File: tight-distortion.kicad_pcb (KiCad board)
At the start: 2 copper layers, 60 x 80 mm, 4 parts, among them J1 Barrel_Jack_Switch, J2 AudioJack_TRS, J3 AudioJack_TRS

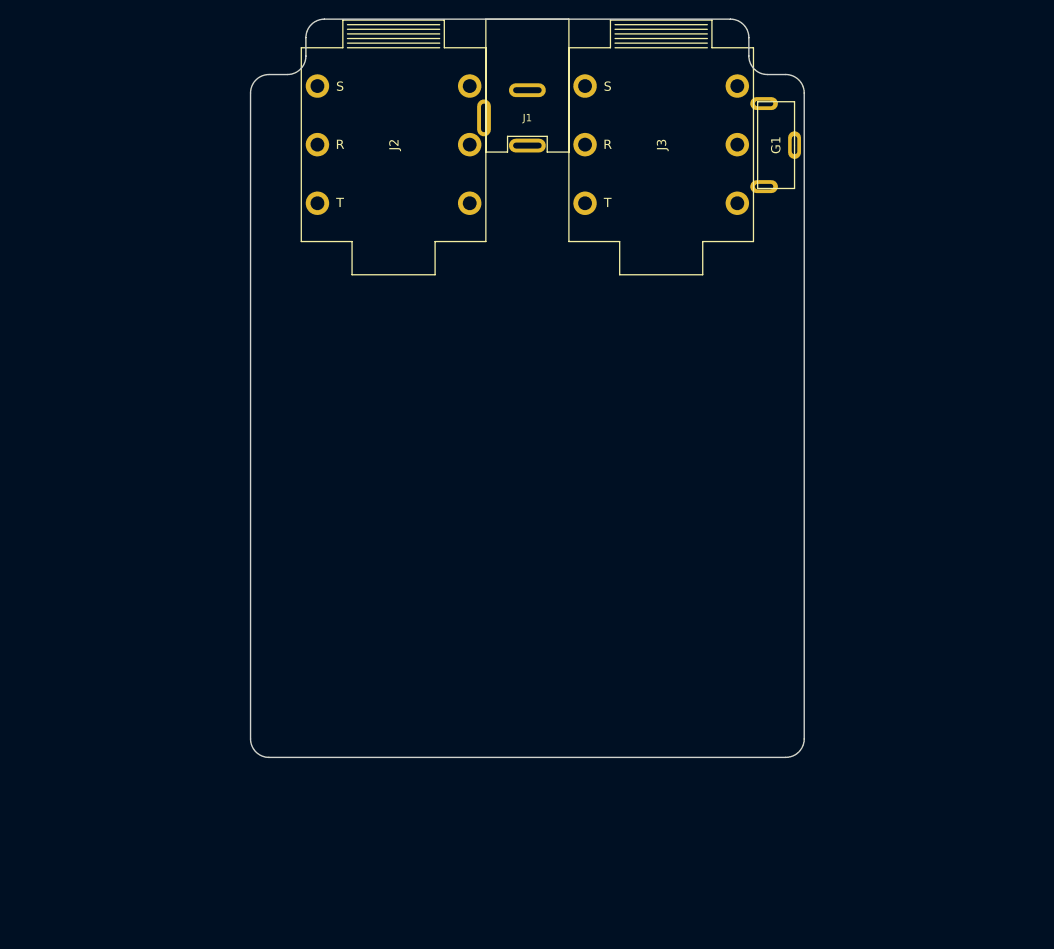
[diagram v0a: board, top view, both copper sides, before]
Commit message: first PCB layout draft
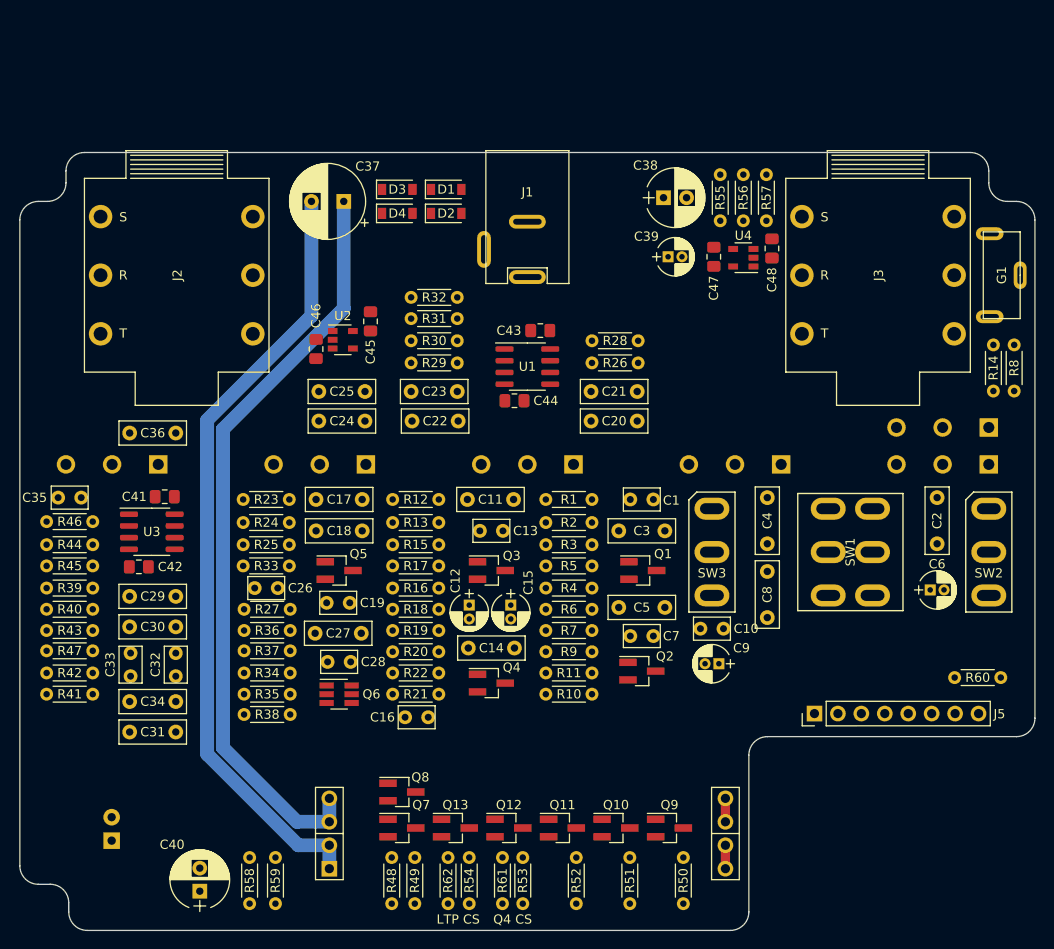
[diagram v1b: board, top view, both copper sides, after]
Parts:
- added C1: 220pF, bca-footprints:C_Ceramic_L4.0mm_W2.5mm_P2.50mm, F.Cu at (12.4, -5.70)
- added C10: 100pF, bca-footprints:C_Ceramic_L4.0mm_W2.5mm_P2.50mm, F.Cu at (20.0, 8.30)
- added C11: 2.2nF, bca-footprints:C_Film_L7.2mm_W2.5mm_P5.00mm, F.Cu at (-4.00, -5.70)
- added C12: 10uF, bca-footprints:CP_Radial_D4.0mm_P1.50mm, F.Cu at (-6.30, 6.50)
- added C13: 100pF, bca-footprints:C_Ceramic_L4.0mm_W2.5mm_P2.50mm, F.Cu at (-3.90, -2.30)
- added C14: 4.7nF, bca-footprints:C_Film_L7.2mm_W2.5mm_P5.00mm, F.Cu at (-3.90, 10.4)
- added C15: 10uF, bca-footprints:CP_Radial_D4.0mm_P1.50mm, F.Cu at (-1.80, 6.50)
- added C16: 100pF, bca-footprints:C_Ceramic_L4.0mm_W2.5mm_P2.50mm, F.Cu at (-12.0, 17.9)
- added C17: 0.1uF, bca-footprints:C_Film_L7.2mm_W2.5mm_P5.00mm, F.Cu at (-20.4, -5.70)
- added C18: 0.1uF, bca-footprints:C_Film_L7.2mm_W2.5mm_P5.00mm, F.Cu at (-20.4, -2.30)
- added C19: 100pF, bca-footprints:C_Ceramic_L4.0mm_W2.5mm_P2.50mm, F.Cu at (-20.5, 5.50)
- added C2: 10nF, bca-footprints:C_Film_L7.2mm_W2.5mm_P5.00mm, F.Cu at (44.4, -3.40)
- added C20: 10nF, bca-footprints:C_Film_L7.2mm_W2.5mm_P5.00mm, F.Cu at (9.40, -14.2)
- added C21: 10nF, bca-footprints:C_Film_L7.2mm_W2.5mm_P5.00mm, F.Cu at (9.40, -17.4)
- added C22: 10nF, bca-footprints:C_Film_L7.2mm_W2.5mm_P5.00mm, F.Cu at (-10.0, -14.2)
- added C23: 10nF, bca-footprints:C_Film_L7.2mm_W2.5mm_P5.00mm, F.Cu at (-10.1, -17.4)
- added C24: 10nF, bca-footprints:C_Film_L7.2mm_W2.5mm_P5.00mm, F.Cu at (-20.1, -14.2)
- added C25: 10nF, bca-footprints:C_Film_L7.2mm_W2.5mm_P5.00mm, F.Cu at (-20.1, -17.4)
- added C26: 100pF, bca-footprints:C_Ceramic_L4.0mm_W2.5mm_P2.50mm, F.Cu at (-28.3, 3.90)
- added C27: 10nF, bca-footprints:C_Film_L7.2mm_W2.5mm_P5.00mm, F.Cu at (-20.5, 8.80)
- added C28: 100pF, bca-footprints:C_Ceramic_L4.0mm_W2.5mm_P2.50mm, F.Cu at (-20.4, 11.9)
- added C29: 0.1uF, bca-footprints:C_Film_L7.2mm_W2.5mm_P5.00mm, F.Cu at (-40.6, 4.80)
- added C3: 1nF, bca-footprints:C_Film_L7.2mm_W2.5mm_P5.00mm, F.Cu at (12.4, -2.30)
- added C30: 0.1uF, bca-footprints:C_Film_L7.2mm_W2.5mm_P5.00mm, F.Cu at (-40.6, 8.10)
- added C31: 0.1uF, bca-footprints:C_Film_L7.2mm_W2.5mm_P5.00mm, F.Cu at (-40.6, 19.5)
- added C32: 270pF, bca-footprints:C_Ceramic_L4.0mm_W2.5mm_P2.50mm, F.Cu at (-38.1, 12.2)
- added C33: 270pF, bca-footprints:C_Ceramic_L4.0mm_W2.5mm_P2.50mm, F.Cu at (-43.0, 12.2)
- added C34: 3.3nF, bca-footprints:C_Film_L7.2mm_W2.5mm_P5.00mm, F.Cu at (-40.6, 16.2)
- added C35: 100pF, bca-footprints:C_Ceramic_L4.0mm_W2.5mm_P2.50mm, F.Cu at (-49.6, -5.90)
- added C36: 0.1uF, bca-footprints:C_Film_L7.2mm_W2.5mm_P5.00mm, F.Cu at (-40.6, -12.9)
- added C37: 470uF, Capacitor_THT:CP_Radial_D8.0mm_P3.50mm, F.Cu at (-19.9, -38.0)
- added C38: 100uF, bca-footprints:CP_Radial_D6.3mm_P2.50mm, F.Cu at (16.0, -38.4)
- added C39: 10uF, bca-footprints:CP_Radial_D4.0mm_P1.50mm, F.Cu at (16.0, -32.0)
- added C4: 22nF, bca-footprints:C_Film_L7.2mm_W2.5mm_P5.00mm, F.Cu at (26.0, -3.40)
- added C40: 100uF, bca-footprints:CP_Radial_D6.3mm_P2.50mm, F.Cu at (-35.5, 35.5)
- added C41: 100nF, Capacitor_SMD:C_0805_2012Metric_Pad1.18x1.45mm_HandSolder, F.Cu at (-39.3, -6.00)
- added C42: 100nF, Capacitor_SMD:C_0805_2012Metric_Pad1.18x1.45mm_HandSolder, F.Cu at (-42.1, 1.60)
- added C43: 100nF, Capacitor_SMD:C_0805_2012Metric_Pad1.18x1.45mm_HandSolder, F.Cu at (1.40, -24.0)
- added C44: 100nF, Capacitor_SMD:C_0805_2012Metric_Pad1.18x1.45mm_HandSolder, F.Cu at (-1.40, -16.4)
- added C45: 100nF, Capacitor_SMD:C_0805_2012Metric_Pad1.18x1.45mm_HandSolder, F.Cu at (-17.0, -25.0)
- added C46: 100nF, Capacitor_SMD:C_0805_2012Metric_Pad1.18x1.45mm_HandSolder, F.Cu at (-22.9, -22.0)
- added C47: 100nF, Capacitor_SMD:C_0805_2012Metric_Pad1.18x1.45mm_HandSolder, F.Cu at (20.2, -32.0)
- added C48: 100nF, Capacitor_SMD:C_0805_2012Metric_Pad1.18x1.45mm_HandSolder, F.Cu at (26.5, -32.9)
- added C5: 2.2nF, bca-footprints:C_Film_L7.2mm_W2.5mm_P5.00mm, F.Cu at (12.4, 6.00)
- added C6: 10uF, bca-footprints:CP_Radial_D4.0mm_P1.50mm, F.Cu at (44.4, 4.10)
- added C7: 470pF, bca-footprints:C_Ceramic_L4.0mm_W2.5mm_P2.50mm, F.Cu at (12.4, 9.10)
- added C8: 2.2nF, bca-footprints:C_Film_L7.2mm_W2.5mm_P5.00mm, F.Cu at (26.0, 4.60)
- added C9: 10uF, bca-footprints:CP_Radial_D4.0mm_P1.50mm, F.Cu at (20.0, 12.1)
- added D1: 1N5819, Diode_SMD:D_SOD-123, F.Cu at (-8.80, -39.3)
- added D2: 1N5819, Diode_SMD:D_SOD-123, F.Cu at (-8.80, -36.7)
- added D3: 1N5819, Diode_SMD:D_SOD-123, F.Cu at (-14.1, -39.3)
- added D4: 1N5819, Diode_SMD:D_SOD-123, F.Cu at (-14.1, -36.7)
- added D5: LED, bca-footprints:LED_D5.0mm, B.Cu at (-45.0, 30.0)
- added J4: power-module, bca-footprints:Power-module, F.Cu at (0.00, 30.5)
- added J5: Conn_01x08, bca-footprints:Pin_Header_Straight_1x08_Pitch2.54mm, F.Cu at (40.0, 17.5)
- added Q1: MMBFJ202, Package_TO_SOT_SMD:SOT-23_Handsoldering, F.Cu at (12.5, 2.00)
- added Q10: BC848C, Package_TO_SOT_SMD:SOT-23_Handsoldering, F.Cu at (9.60, 29.9)
- added Q11: BC848C, Package_TO_SOT_SMD:SOT-23_Handsoldering, F.Cu at (3.80, 29.9)
- added Q12: BC848C, Package_TO_SOT_SMD:SOT-23_Handsoldering, F.Cu at (-2.00, 29.9)
- added Q13: BC848C, Package_TO_SOT_SMD:SOT-23_Handsoldering, F.Cu at (-7.80, 29.9)
- added Q2: MMBFJ202, Package_TO_SOT_SMD:SOT-23_Handsoldering, F.Cu at (12.4, 12.9)
- added Q3: MMBFJ202, Package_TO_SOT_SMD:SOT-23_Handsoldering, F.Cu at (-3.90, 2.00)
- added Q4: MMBFJ202, Package_TO_SOT_SMD:SOT-23_Handsoldering, F.Cu at (-3.90, 14.2)
- added Q5: BC848C, Package_TO_SOT_SMD:SOT-23_Handsoldering, F.Cu at (-20.4, 2.00)
- added Q6: LS844, Package_TO_SOT_SMD:SOT-23-6_Handsoldering, F.Cu at (-20.4, 15.4)
- added Q7: BC848C, Package_TO_SOT_SMD:SOT-23_Handsoldering, F.Cu at (-13.6, 29.9)
- added Q8: BC848C, Package_TO_SOT_SMD:SOT-23_Handsoldering, F.Cu at (-13.6, 26.0)
- added Q9: BC848C, Package_TO_SOT_SMD:SOT-23_Handsoldering, F.Cu at (15.4, 29.9)
- added R1: 68k, bca-footprints:R_L3.6mm_D1.6mm_P5.00mm_Horizontal, F.Cu at (4.50, -5.70)
- added R10: 15k, bca-footprints:R_L3.6mm_D1.6mm_P5.00mm_Horizontal, F.Cu at (4.50, 15.4)
- added R11: 2k, bca-footprints:R_L3.6mm_D1.6mm_P5.00mm_Horizontal, F.Cu at (4.50, 13.1)
- added R12: 220k, bca-footprints:R_L3.6mm_D1.6mm_P5.00mm_Horizontal, F.Cu at (-12.1, -5.70)
- added R13: 470k, bca-footprints:R_L3.6mm_D1.6mm_P5.00mm_Horizontal, F.Cu at (-12.1, -3.20)
- added R14: 47k, bca-footprints:R_L3.6mm_D1.6mm_P5.00mm_Horizontal, F.Cu at (50.5, -19.9)
- added R15: 47k, bca-footprints:R_L3.6mm_D1.6mm_P5.00mm_Horizontal, F.Cu at (-12.1, -0.80)
- added R16: 15k, bca-footprints:R_L3.6mm_D1.6mm_P5.00mm_Horizontal, F.Cu at (-12.1, 3.90)
- added R17: 2k, bca-footprints:R_L3.6mm_D1.6mm_P5.00mm_Horizontal, F.Cu at (-12.1, 1.50)
- added R18: 470k, bca-footprints:R_L3.6mm_D1.6mm_P5.00mm_Horizontal, F.Cu at (-12.1, 6.20)
- added R19: 220k, bca-footprints:R_L3.6mm_D1.6mm_P5.00mm_Horizontal, F.Cu at (-12.1, 8.50)
- added R2: 1M, bca-footprints:R_L3.6mm_D1.6mm_P5.00mm_Horizontal, F.Cu at (4.50, -3.20)
- added R20: 47k, bca-footprints:R_L3.6mm_D1.6mm_P5.00mm_Horizontal, F.Cu at (-12.1, 10.8)
- added R21: 7.5k, bca-footprints:R_L3.6mm_D1.6mm_P5.00mm_Horizontal, F.Cu at (-12.1, 15.4)
- added R22: 1k, bca-footprints:R_L3.6mm_D1.6mm_P5.00mm_Horizontal, F.Cu at (-12.1, 13.1)
- added R23: 470k, bca-footprints:R_L3.6mm_D1.6mm_P5.00mm_Horizontal, F.Cu at (-28.3, -5.70)
- added R24: 100k, bca-footprints:R_L3.6mm_D1.6mm_P5.00mm_Horizontal, F.Cu at (-28.3, -3.20)
- added R25: 15k, bca-footprints:R_L3.6mm_D1.6mm_P5.00mm_Horizontal, F.Cu at (-28.3, -0.80)
- added R26: 2k, bca-footprints:R_L3.6mm_D1.6mm_P5.00mm_Horizontal, F.Cu at (9.50, -20.5)
- added R27: 10k, bca-footprints:R_L3.6mm_D1.6mm_P5.00mm_Horizontal, F.Cu at (-28.2, 6.20)
- added R28: 2k, bca-footprints:R_L3.6mm_D1.6mm_P5.00mm_Horizontal, F.Cu at (9.50, -22.9)
- added R29: 2k, bca-footprints:R_L3.6mm_D1.6mm_P5.00mm_Horizontal, F.Cu at (-10.1, -20.5)
- added R3: 1M, bca-footprints:R_L3.6mm_D1.6mm_P5.00mm_Horizontal, F.Cu at (4.50, -0.80)
- added R30: 2k, bca-footprints:R_L3.6mm_D1.6mm_P5.00mm_Horizontal, F.Cu at (-10.1, -22.9)
- added R31: 2k, bca-footprints:R_L3.6mm_D1.6mm_P5.00mm_Horizontal, F.Cu at (-10.1, -25.3)
- added R32: 2k, bca-footprints:R_L3.6mm_D1.6mm_P5.00mm_Horizontal, F.Cu at (-10.1, -27.6)
- added R33: 10k, bca-footprints:R_L3.6mm_D1.6mm_P5.00mm_Horizontal, F.Cu at (-28.3, 1.50)
- added R34: 1M, bca-footprints:R_L3.6mm_D1.6mm_P5.00mm_Horizontal, F.Cu at (-28.2, 13.1)
- added R35: 10k, bca-footprints:R_L3.6mm_D1.6mm_P5.00mm_Horizontal, F.Cu at (-28.2, 15.4)
- added R36: 15k, bca-footprints:R_L3.6mm_D1.6mm_P5.00mm_Horizontal, F.Cu at (-28.2, 8.50)
- added R37: 15k, bca-footprints:R_L3.6mm_D1.6mm_P5.00mm_Horizontal, F.Cu at (-28.2, 10.7)
- added R38: 1M, bca-footprints:R_L3.6mm_D1.6mm_P5.00mm_Horizontal, F.Cu at (-28.2, 17.6)
- added R39: 100k, bca-footprints:R_L3.6mm_D1.6mm_P5.00mm_Horizontal, F.Cu at (-49.6, 3.90)
- added R4: 15k, bca-footprints:R_L3.6mm_D1.6mm_P5.00mm_Horizontal, F.Cu at (4.50, 3.90)
- added R40: 100k, bca-footprints:R_L3.6mm_D1.6mm_P5.00mm_Horizontal, F.Cu at (-49.6, 6.20)
- added R41: 10k, bca-footprints:R_L3.6mm_D1.6mm_P5.00mm_Horizontal, F.Cu at (-49.6, 15.4)
- added R42: 470R, bca-footprints:R_L3.6mm_D1.6mm_P5.00mm_Horizontal, F.Cu at (-49.6, 13.1)
- added R43: 100k, bca-footprints:R_L3.6mm_D1.6mm_P5.00mm_Horizontal, F.Cu at (-49.6, 8.50)
- added R44: 10k, bca-footprints:R_L3.6mm_D1.6mm_P5.00mm_Horizontal, F.Cu at (-49.6, -0.80)
- added R45: 10k, bca-footprints:R_L3.6mm_D1.6mm_P5.00mm_Horizontal, F.Cu at (-49.6, 1.50)
- added R46: 100k, bca-footprints:R_L3.6mm_D1.6mm_P5.00mm_Horizontal, F.Cu at (-49.6, -3.30)
- added R47: 100k, bca-footprints:R_L3.6mm_D1.6mm_P5.00mm_Horizontal, F.Cu at (-49.6, 10.7)
- added R48: 27k, bca-footprints:R_L3.6mm_D1.6mm_P5.00mm_Horizontal, F.Cu at (-14.7, 35.6)
- added R49: 470R, bca-footprints:R_L3.6mm_D1.6mm_P5.00mm_Horizontal, F.Cu at (-12.2, 35.6)
- added R5: 2k, bca-footprints:R_L3.6mm_D1.6mm_P5.00mm_Horizontal, F.Cu at (4.50, 1.50)
- added R50: 470R, bca-footprints:R_L3.6mm_D1.6mm_P5.00mm_Horizontal, F.Cu at (16.9, 35.6)
- added R51: 470R, bca-footprints:R_L3.6mm_D1.6mm_P5.00mm_Horizontal, F.Cu at (11.1, 35.6)
- added R52: 470R, bca-footprints:R_L3.6mm_D1.6mm_P5.00mm_Horizontal, F.Cu at (5.30, 35.6)
- added R53: 470R, bca-footprints:R_L3.6mm_D1.6mm_P5.00mm_Horizontal, F.Cu at (-0.50, 35.6)
- added R54: 470R, bca-footprints:R_L3.6mm_D1.6mm_P5.00mm_Horizontal, F.Cu at (-6.30, 35.6)
- added R55: 1k, bca-footprints:R_L3.6mm_D1.6mm_P5.00mm_Horizontal, F.Cu at (20.9, -38.4)
- added R56: 2k, bca-footprints:R_L3.6mm_D1.6mm_P5.00mm_Horizontal, F.Cu at (23.4, -38.4)
- added R57: 12k, bca-footprints:R_L3.6mm_D1.6mm_P5.00mm_Horizontal, F.Cu at (25.9, -38.4)
- added R58: 12k, bca-footprints:R_L3.6mm_D1.6mm_P5.00mm_Horizontal, F.Cu at (-30.1, 35.6)
- added R59: 3.3k, bca-footprints:R_L3.6mm_D1.6mm_P5.00mm_Horizontal, F.Cu at (-27.3, 35.6)
- added R6: 220k, bca-footprints:R_L3.6mm_D1.6mm_P5.00mm_Horizontal, F.Cu at (4.50, 6.20)
- added R60: 33k, bca-footprints:R_L3.6mm_D1.6mm_P5.00mm_Horizontal, F.Cu at (48.8, 13.6)
- added R61: 470R, bca-footprints:R_L3.6mm_D1.6mm_P5.00mm_Horizontal, F.Cu at (-2.70, 35.6)
- added R62: 470R, bca-footprints:R_L3.6mm_D1.6mm_P5.00mm_Horizontal, F.Cu at (-8.60, 35.6)
- added R7: 220k, bca-footprints:R_L3.6mm_D1.6mm_P5.00mm_Horizontal, F.Cu at (4.50, 8.50)
- added R8: 47k, bca-footprints:R_L3.6mm_D1.6mm_P5.00mm_Horizontal, F.Cu at (52.8, -19.9)
- added R9: 47k, bca-footprints:R_L3.6mm_D1.6mm_P5.00mm_Horizontal, F.Cu at (4.50, 10.8)
- added RV1: 500kA, bca-footprints:R_POT_DUAL, F.Cu at (45.0, -26.0)
- added RV2: 100kB, bca-footprints:R_POT, F.Cu at (22.5, -26.0)
- added RV3: 100kB, bca-footprints:R_POT, F.Cu at (0.00, -26.0)
- added RV4: 100kB, bca-footprints:R_POT, F.Cu at (-22.5, -26.0)
- added RV5: 100kA, bca-footprints:R_POT, F.Cu at (-45.0, -26.0)
- added SW1: SW_DPDT_x2, bca-footprints:SW_Toggle_DPDT_SolderLug, F.Cu at (35.0, 0.00)
- added SW2: SW_SPDT, bca-footprints:SW_Toggle_SPDT_SolderLug, F.Cu at (50.0, 0.00)
- added SW3: SW_SPDT, bca-footprints:SW_Toggle_SPDT_SolderLug, F.Cu at (20.0, 0.00)
- added U1: TLV9302, Package_SO:SOIC-8_3.9x4.9mm_P1.27mm, F.Cu at (0.00, -20.1)
- added U2: TLV9301, Package_TO_SOT_SMD:SOT-23-5, F.Cu at (-20.0, -23.0)
- added U3: OPA1692xD, Package_SO:SOIC-8_3.9x4.9mm_P1.27mm, F.Cu at (-40.7, -2.20)
- added U4: TLV9301, Package_TO_SOT_SMD:SOT-23-5, F.Cu at (23.4, -31.9)
- moved G1 28.2 mm to (53.4, -30.0)
- moved J2 27.4 mm to (-38.0, -30.0)
- moved J3 27.4 mm to (38.0, -30.0)
- moved J1 14.2 mm to (0.00, -43.5)
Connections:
- J1 pad 1: Net-(J1-Pad1) -> Net-(D2-Pad1)
- J2 pad 2: Net-(J1-Pad1) -> Earth
- J2 pad 5: Net-(J2-Pad5) -> Earth
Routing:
- net Earth: track 0.00 -> 84.5 mm
- net Net-(C37-Pad1): track 0.00 -> 82.0 mm
- net -15V: track 0.00 -> 2.54 mm
- net +15V: track 0.00 -> 2.54 mm
- added copper zone on In1.Cu, net Earth
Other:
- board size 60 x 80 mm -> 110 x 84.3 mm
- copper layers 2 -> 4
- net class Default: trace_width 0.15 -> 0.25
- net class PWR removed
- rule trace_min: 0.15 -> 0.2
- rule via_min_drill: 0.4 -> 0.3
- rule via_min_size: 0.8 -> 0.4
- board text added: "JLCJLCJLCJLC"
- board text added: "LTP CS"
- board text added: "Q4 CS"
